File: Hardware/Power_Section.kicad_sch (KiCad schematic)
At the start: 39 parts, among them IC1 TPS54202HDDCR, Q1 SI2347DS-T1-GE3, U1 TLV743P, U2 TLV743P, U3 TLV743P, U4 TLV743P

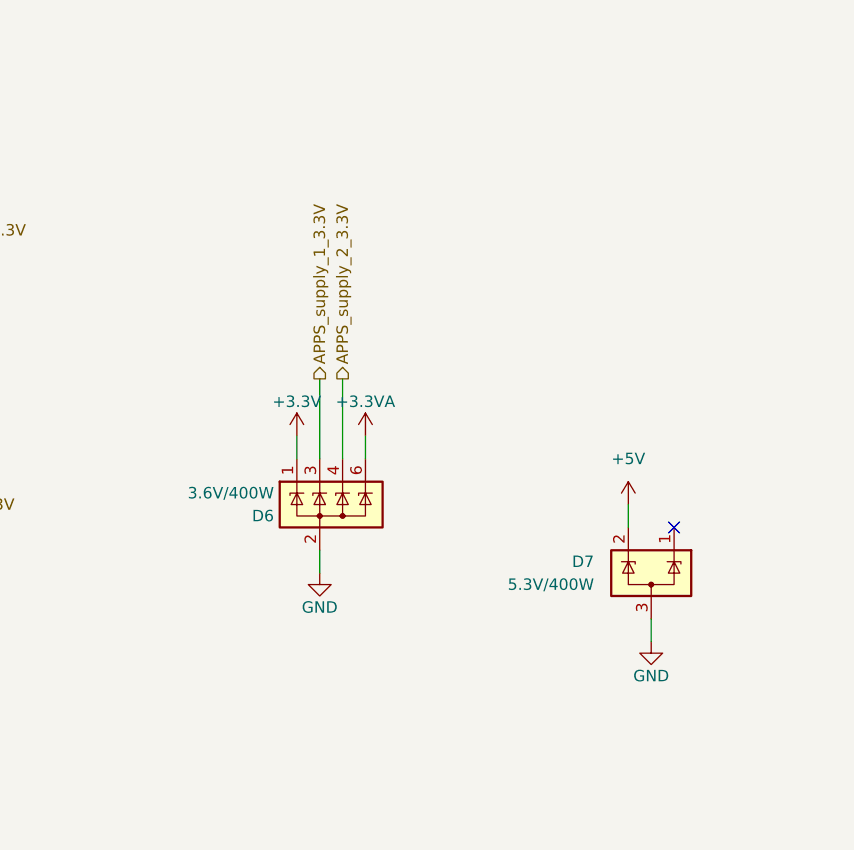
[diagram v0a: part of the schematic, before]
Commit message: Changes in CAN section
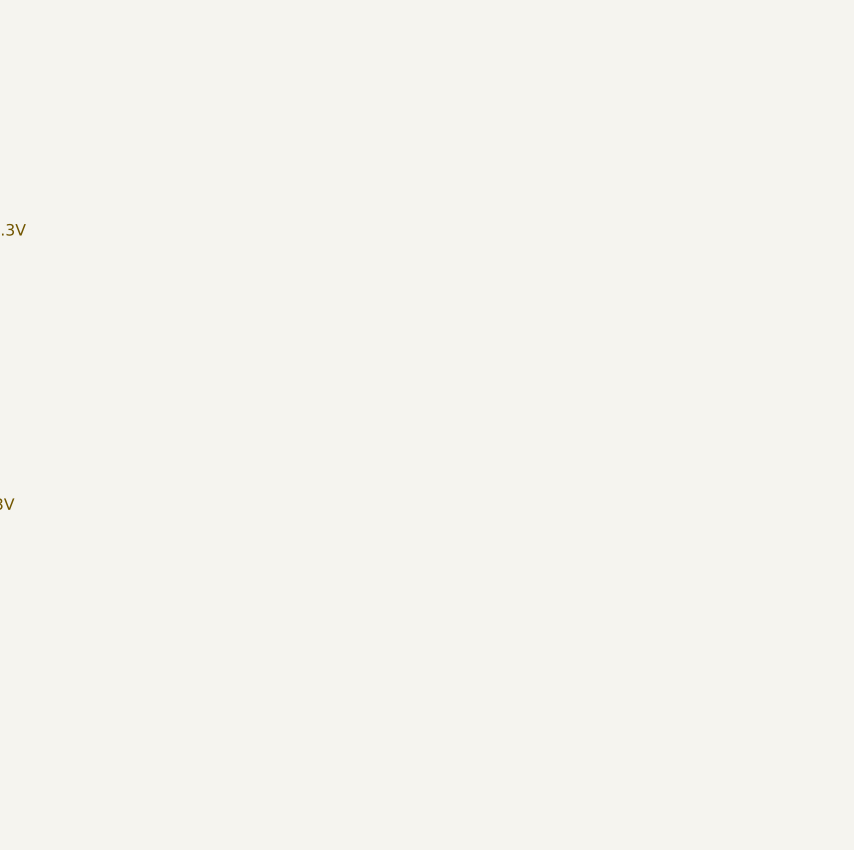
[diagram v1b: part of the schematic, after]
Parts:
- removed D6: 3.6V/400W, Package_TO_SOT_SMD:SOT-23-6, symbol Power_Protection:ESDA5V3SC5
- removed D7: 5.3V/400W, Package_TO_SOT_SMD:SOT-23-3, symbol Power_Protection:ESDA5V3L
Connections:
- no-connect marks 1 -> 0
